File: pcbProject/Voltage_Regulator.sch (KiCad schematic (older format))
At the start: 4 parts, among them U1 NCP1117

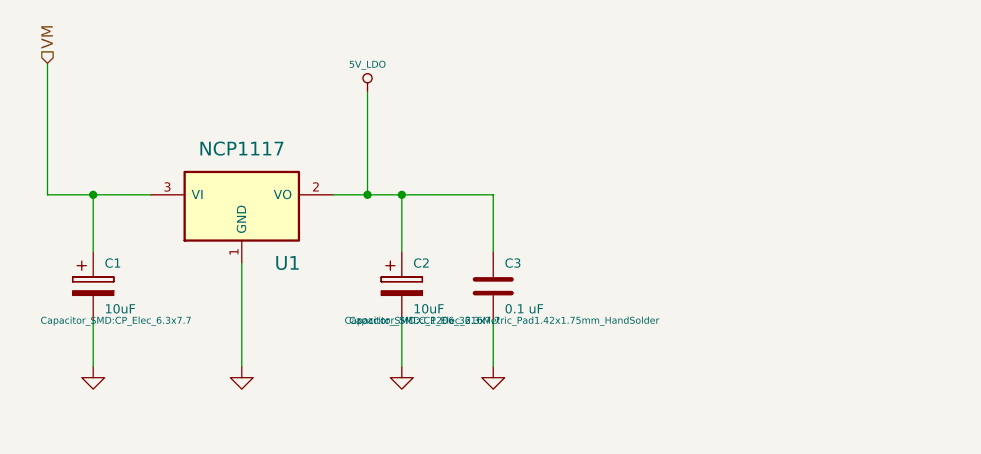
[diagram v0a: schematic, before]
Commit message: verslag
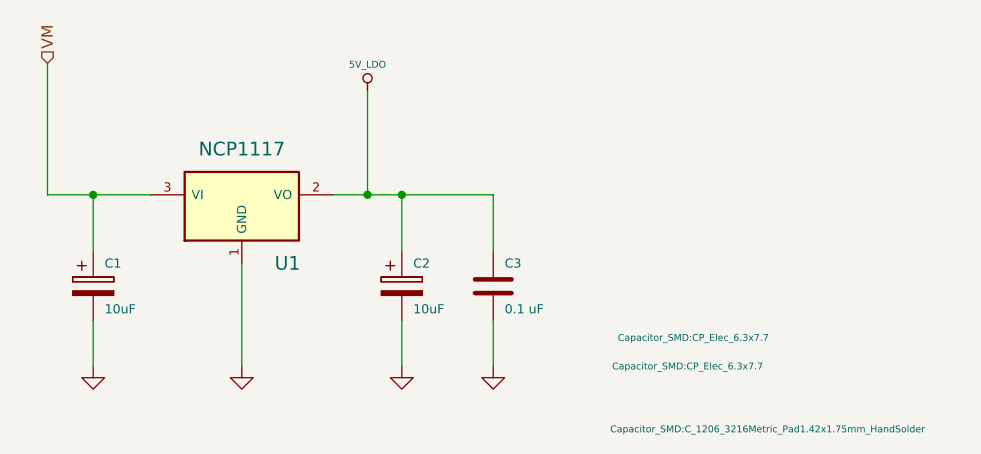
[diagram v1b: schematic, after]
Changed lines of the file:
@@
 F 0 "C1" H 5325 4275 40  0000 L CNN
 F 1 "10uF" H 5325 4075 40  0000 L CNN
-F 2 "Capacitor_SMD:CP_Elec_6.3x7.7" H 5375 4025 30  0000 C CNN
+F 2 "Capacitor_SMD:CP_Elec_6.3x7.7" H 7900 3950 30  0000 C CNN
 F 3 "http://images.ihscontent.net/vipimages/VipMasterIC/IC/BEYS/BEYSS04513/BEYSS04513-1.pdf" H 5275 4175 300 0001 C CNN
 F 4 "CAPACITOR, ALUMINUM ELECTROLYTIC, NON SOLID, POLARIZED, 50 V, 47 uF, SURFACE MOUNT, 3131, CHIP, ROHS COMPLIANT" H 5275 4175 60  0001 C CNN "Characteristics"
@@
 F 0 "C3" H 7075 4275 40  0000 L CNN
 F 1 "0.1 uF" H 7075 4075 40  0000 L CNN
-F 2 "Capacitor_SMD:C_1206_3216Metric_Pad1.42x1.75mm_HandSolder" H 7063 4025 30  0000 C CNN
+F 2 "Capacitor_SMD:C_1206_3216Metric_Pad1.42x1.75mm_HandSolder" H 8225 3550 30  0000 C CNN
 F 3 "http://images.ihscontent.net/vipimages/VipMasterIC/IC/KEME/KEMES10043/KEMES10043-1.pdf" H 7025 4175 60  0001 C CNN
 F 4 "CAPACITOR, CERAMIC, MULTILAYER, 100 V, X7R, 0.1 uF, SURFACE MOUNT, 0805, CHIP, ROHS COMPLIANT" H 7025 4175 60  0001 C CNN "Characteristics"
@@
 F 0 "C2" H 6675 4275 40  0000 L CNN
 F 1 "10uF" H 6675 4075 40  0000 L CNN
-F 2 "Capacitor_SMD:CP_Elec_6.3x7.7" H 6725 4025 30  0000 C CNN
+F 2 "Capacitor_SMD:CP_Elec_6.3x7.7" H 7875 3825 30  0000 C CNN
 F 3 "http://images.ihscontent.net/vipimages/VipMasterIC/IC/BEYS/BEYSS04513/BEYSS04513-1.pdf" H 6625 4175 300 0001 C CNN
 F 4 "CAPACITOR, ALUMINUM ELECTROLYTIC, NON SOLID, POLARIZED, 50 V, 47 uF, SURFACE MOUNT, 3131, CHIP, ROHS COMPLIANT" H 6625 4175 60  0001 C CNN "Characteristics"
